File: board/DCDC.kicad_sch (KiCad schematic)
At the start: 30 parts, among them U1 TPS65131

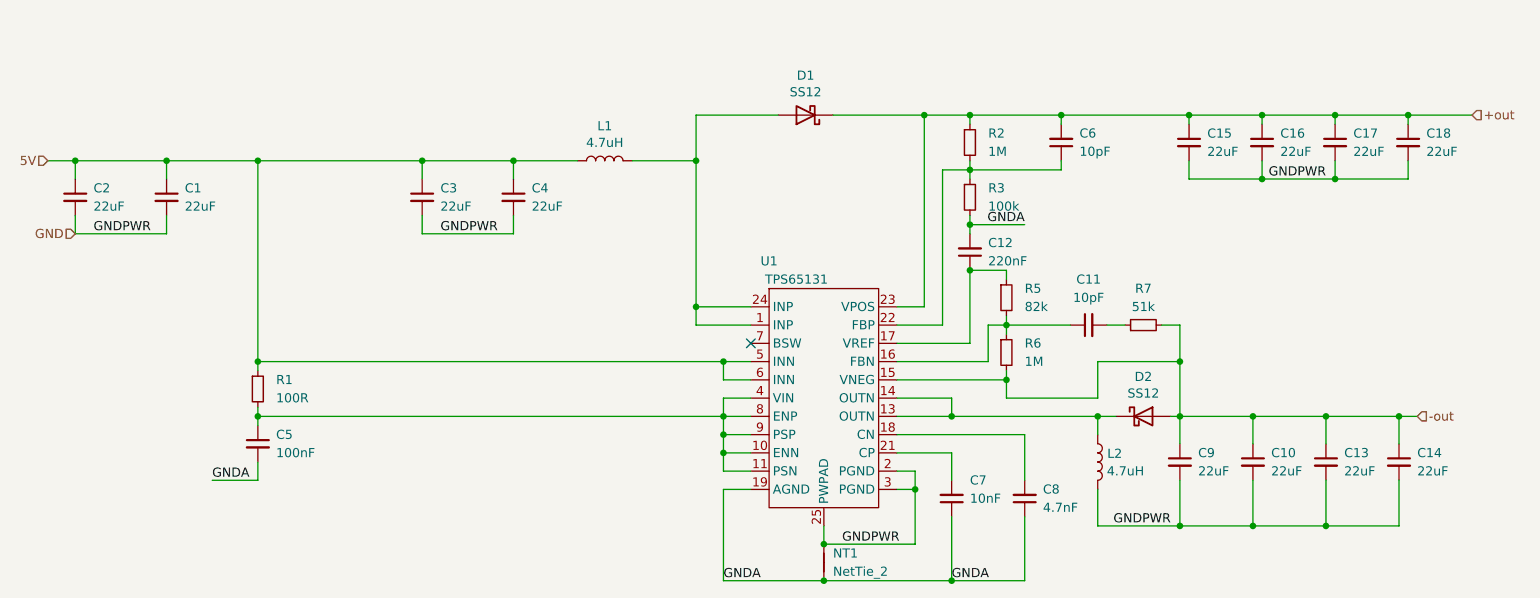
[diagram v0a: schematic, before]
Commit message: initial b146
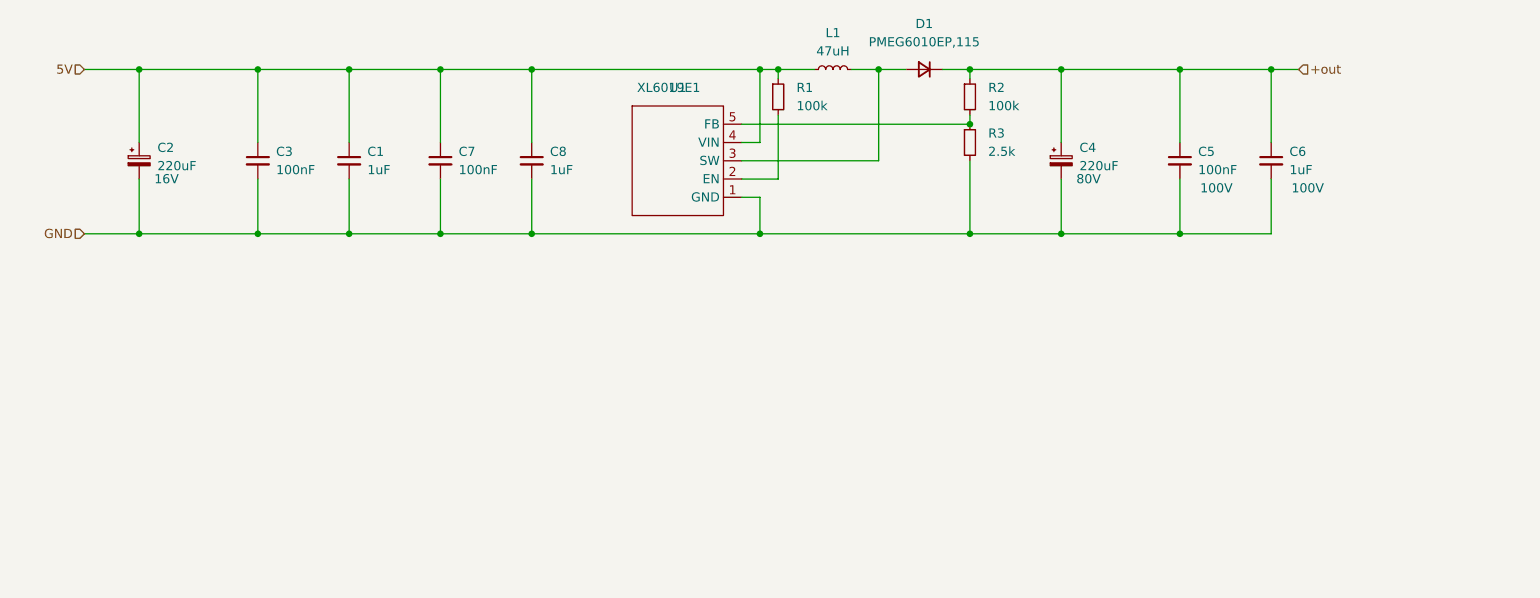
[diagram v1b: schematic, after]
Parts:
- removed C10, C13, C14, C15, C16, C17, C18, C2, C4, C9: 22uF, Capacitor_SMD:C_0805_2012Metric, symbol Device:C_Small
- removed C11: 10pF, Capacitor_SMD:C_0402_1005Metric, symbol Device:C_Small
- removed C12: 220nF, Capacitor_SMD:C_0402_1005Metric, symbol Device:C_Small
- removed D1, D2: SS12, Diode_SMD:D_SMA, symbol Device:D_Schottky
- removed L1, L2: 4.7uH, Inductor_SMD:L_6.3x6.3_H3, symbol Device:L
- removed NT1: NetTie_2, NetTie:NetTie-2_SMD_Pad0.5mm, symbol Device:NetTie_2
- removed R5: 82k, Resistor_SMD:R_0402_1005Metric, symbol Device:R_Small
- removed R6: 1M, Resistor_SMD:R_0402_1005Metric, symbol Device:R_Small
- removed R7: 51k, Resistor_SMD:R_0402_1005Metric, symbol Device:R_Small
- removed U1: TPS65131, Package_DFN_QFN:VQFN-24-1EP_4x4mm_P0.5mm_EP2.45x2.45mm_ThermalVias, symbol b145:TPS65130/1
- added C2, C4: 220uF, Capacitor_SMD:CP_Elec_10x14.3, symbol Device:C_Polarized_Small
- added D1: PMEG6010EP,115, Diode_SMD:D_SOD-128, symbol Device:D_Small
- added L1: 47uH, Inductor_SMD:L_Sunlord_MWSA1206S-470, symbol Device:L_Small
- added U1: XL6019E1, Package_TO_SOT_SMD:TO-263-5_TabPin3, symbol b146:XL6019E1
- C1: value 22uF -> 1uF; footprint Capacitor_SMD:C_0805_2012Metric -> Capacitor_SMD:C_0603_1608Metric
- C3: value 22uF -> 100nF; footprint Capacitor_SMD:C_0805_2012Metric -> Capacitor_SMD:C_0603_1608Metric
- C5: footprint Capacitor_SMD:C_0402_1005Metric -> Capacitor_SMD:C_0603_1608Metric; Voltage (none) -> 100V
- C6: value 10pF -> 1uF; footprint Capacitor_SMD:C_0402_1005Metric -> Capacitor_SMD:C_1206_3216Metric; Voltage (none) -> 100V
- C7: value 10nF -> 100nF; footprint Capacitor_SMD:C_0402_1005Metric -> Capacitor_SMD:C_0603_1608Metric
- C8: value 4.7nF -> 1uF; footprint Capacitor_SMD:C_0402_1005Metric -> Capacitor_SMD:C_0603_1608Metric
- R1: value 100R -> 100k
- R2: value 1M -> 100k; footprint Resistor_SMD:R_0402_1005Metric -> Resistor_SMD:R_0603_1608Metric
- R3: value 100k -> 2.5k; footprint Resistor_SMD:R_0402_1005Metric -> Resistor_SMD:R_0603_1608Metric
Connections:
- net +out: now also C5.1, C6.1, C4.1, D1.1 (K); no longer C6.2
- net 5V: now also C7.1, C8.1, C2.1, L1.1, U1.4 (VIN)
- net GND: now also C5.2, C6.2, C7.2, C8.2, R3.2, C2.2, C4.2, U1.1 (GND)
- net at R2.2, R3.1: now also U1.5 (FB); no longer C6.1
- net at R1.2: now also U1.2 (EN); no longer C5.1
- removed net GNDA: C5.2, C7.1, C8.1, R3.2
- new net: D1.2 (A), L1.2, U1.3 (SW)
- no-connect marks 1 -> 0
